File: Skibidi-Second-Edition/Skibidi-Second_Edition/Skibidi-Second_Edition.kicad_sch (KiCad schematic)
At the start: 72 parts, among them IC1 TEENSY_4.1, J1 Screw_Terminal_01x03, J10 Screw_Terminal_01x03, J11 Screw_Terminal_01x03, J12 12V, J13 Conn_01x03_Pin, J14 Conn_01x08_Pin, J15 Conn_02x05_Odd_Even, J16 P78E05-1000, J17 Conn_01x04_Pin, J2 Screw_Terminal_01x03, J3 Screw_Terminal_01x03, J4 Screw_Terminal_01x03, J5 Screw_Terminal_01x03, J6 Screw_Terminal_01x03, J7 Screw_Terminal_01x03, J8 Screw_Terminal_01x03, J9 Screw_Terminal_01x03, SW1 SW_Nidec_CAS-120A1, SW2 210-4MS

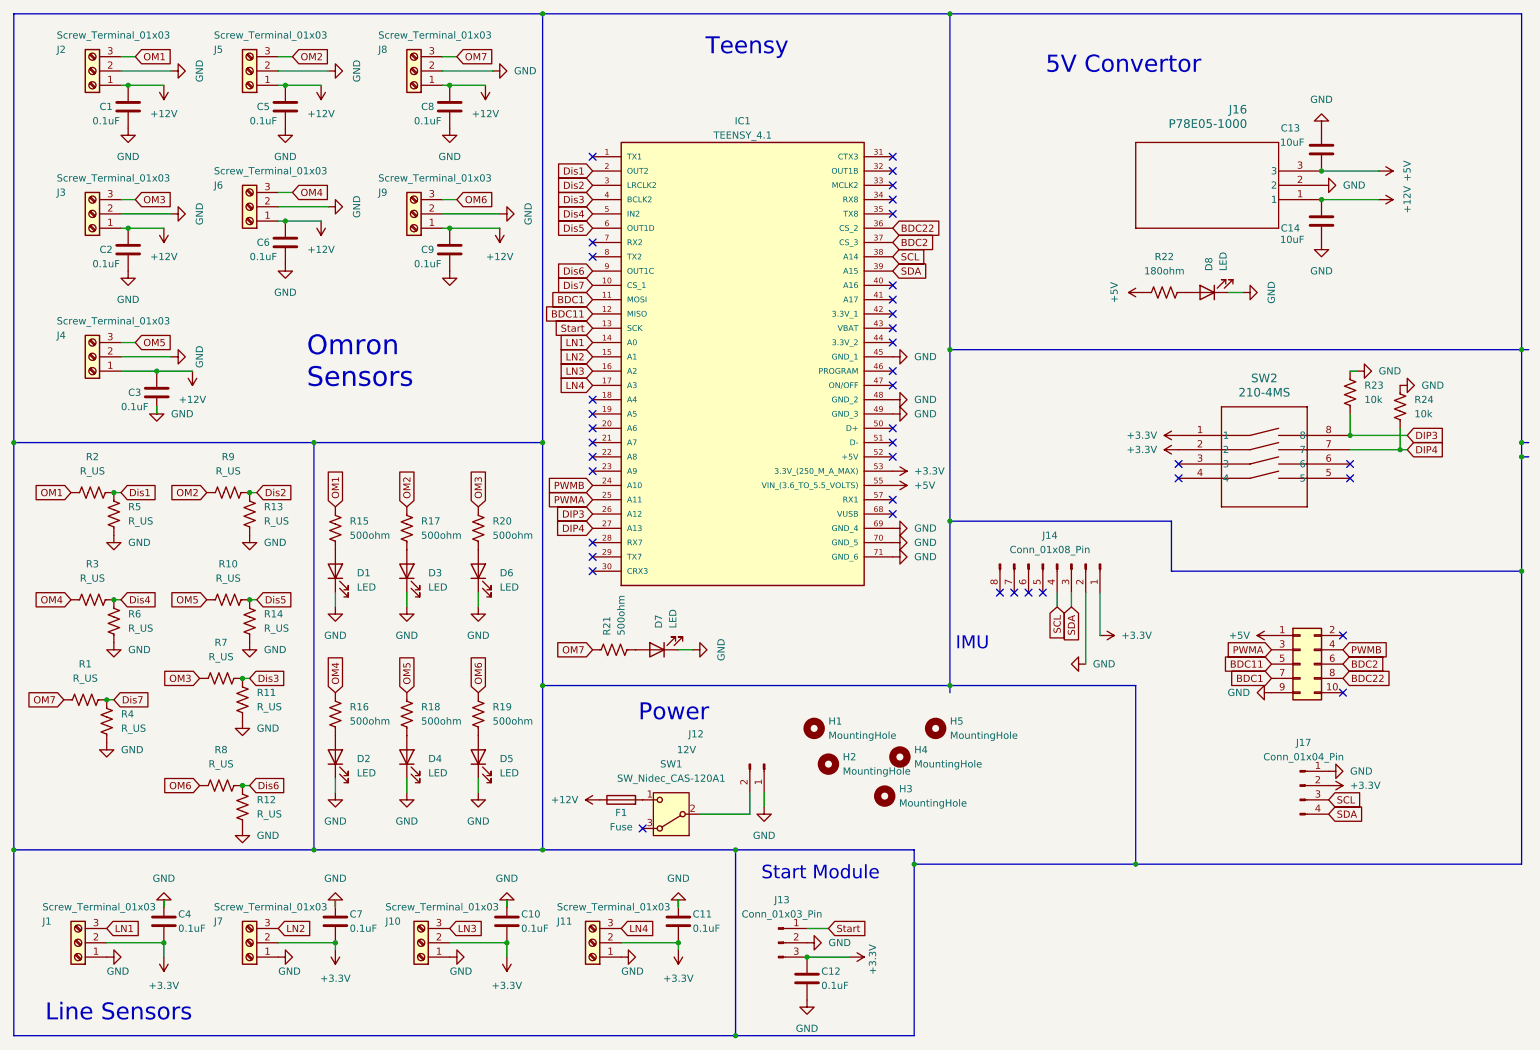
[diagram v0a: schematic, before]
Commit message: skibidi
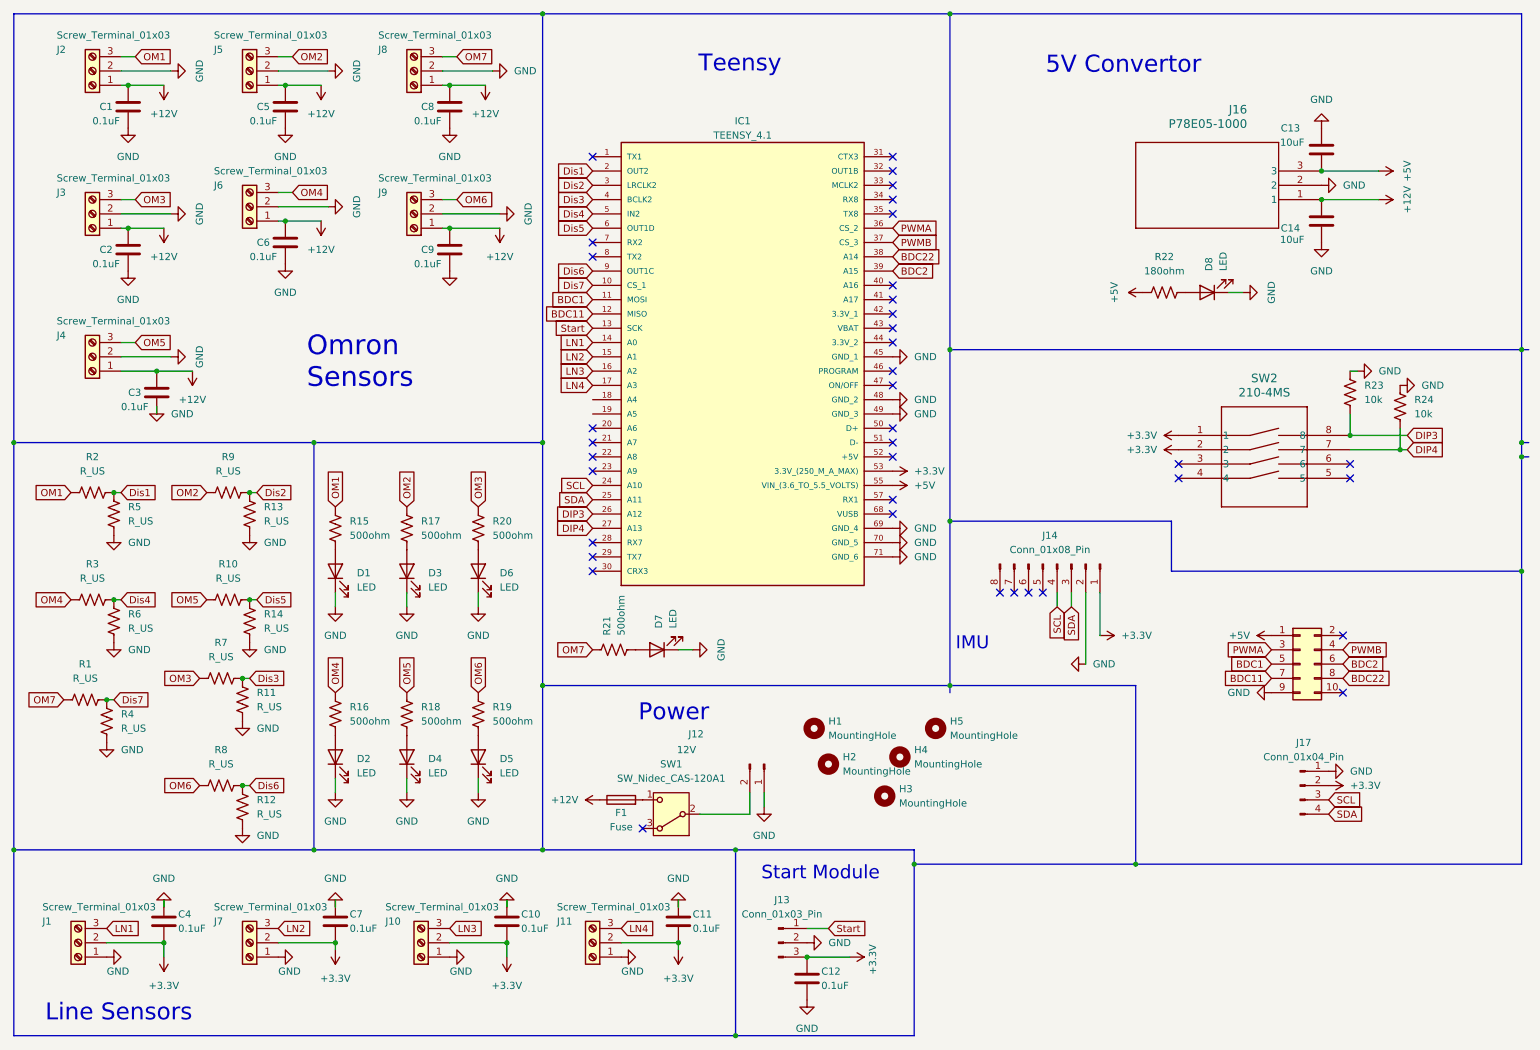
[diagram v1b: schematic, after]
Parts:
- J1, J10, J11, J2, J3, J4, J5, J6, J7, J8, J9: footprint TerminalBlock:TerminalBlock_Xinya_XY308-2.54-3P_1x03_P2.54mm_Horizontal -> Connector_JST:JST_EH_B3B-EH-A_1x03_P2.50mm_Vertical
- J17: footprint (none) -> Connector_PinHeader_2.54mm:PinHeader_1x04_P2.54mm_Vertical
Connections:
- net BDC1: now also J15.5 (Pin_5); no longer J15.7 (Pin_7)
- net BDC11: now also J15.7 (Pin_7); no longer J15.5 (Pin_5)
- net BDC2: now also IC1.39 (A15); no longer IC1.37 (CS_3)
- net BDC22: now also IC1.38 (A14); no longer IC1.36 (CS_2)
- net PWMA: now also IC1.36 (CS_2); no longer IC1.25 (A11)
- net PWMB: now also IC1.37 (CS_3); no longer IC1.24 (A10)
- net SCL: now also IC1.24 (A10); no longer IC1.38 (A14)
- net SDA: now also IC1.25 (A11); no longer IC1.39 (A15)
- no-connect marks 40 -> 38
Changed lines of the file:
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@@
 	)
 	(no_connect
-		(at 118.11 83.82)
-	)
-	(no_connect
 		(at 171.45 63.5)
 	)
@@
 	)
 	(no_connect
-		(at 118.11 81.28)
-	)
-	(no_connect
 		(at 118.11 53.34)
 	)
@@
 	(text "Teensy\n"
 		(exclude_from_sim no)
-		(at 138.176 20.32 0)
+		(at 136.906 23.368 0)
 		(effects
 			(font
@@
 		)
 	)
+	(global_label "PWMB"
+		(shape input)
+		(at 171.45 53.34 0)
+		(fields_autoplaced yes)
+		(effects
+			(font
+				(size 1.27 1.27)
+			)
+			(justify left)
+		)
+		(property "Intersheetrefs" "${INTERSHEET_REFS}"
+			(at 179.878 53.34 0)
+			(effects
+				(font
+					(size 1.27 1.27)
+				)
+				(justify left)
+				(hide yes)
+			)
+		)
+	)
 	(global_label "Dis1"
 		(shape input)
@@
 		)
 	)
+	(global_label "PWMA"
+		(shape input)
+		(at 171.45 50.8 0)
+		(fields_autoplaced yes)
+		(effects
+			(font
+				(size 1.27 1.27)
+			)
+			(justify left)
+		)
+		(property "Intersheetrefs" "${INTERSHEET_REFS}"
+			(at 179.6966 50.8 0)
+			(effects
+				(font
+					(size 1.27 1.27)
+				)
+				(justify left)
+				(hide yes)
+			)
+		)
+	)
+	(global_label "SCL"
+		(shape input)
+		(at 118.11 96.52 180)
+		(fields_autoplaced yes)
+		(effects
+			(font
+				(size 1.27 1.27)
+			)
+			(justify right)
+		)
+		(property "Intersheetrefs" "${INTERSHEET_REFS}"
+			(at 111.6172 96.52 0)
+			(effects
+				(font
+					(size 1.27 1.27)
+				)
+				(justify right)
+				(hide yes)
+			)
+		)
+	)
 	(global_label "SCL"
 		(shape input)
@@
 		)
 	)
-	(global_label "BDC2"
-		(shape input)
-		(at 171.45 53.34 0)
-		(fields_autoplaced yes)
-		(effects
-			(font
-				(size 1.27 1.27)
-			)
-			(justify left)
-		)
-		(property "Intersheetrefs" "${INTERSHEET_REFS}"
-			(at 179.4547 53.34 0)
-			(effects
-				(font
-					(size 1.27 1.27)
-				)
-				(justify left)
-				(hide yes)
-			)
-		)
-	)
 	(global_label "Dis4"
 		(shape input)
@@
 		)
 	)
-	(global_label "BDC11"
+	(global_label "BDC1"
 		(shape input)
 		(at 238.76 128.27 180)
@@
 		)
 		(property "Intersheetrefs" "${INTERSHEET_REFS}"
-			(at 229.5458 128.27 0)
+			(at 230.7553 128.27 0)
 			(effects
 				(font
@@
 		)
 	)
-	(global_label "BDC1"
+	(global_label "BDC11"
 		(shape input)
 		(at 238.76 130.81 180)
@@
 		)
 		(property "Intersheetrefs" "${INTERSHEET_REFS}"
-			(at 230.7553 130.81 0)
+			(at 229.5458 130.81 0)
 			(effects
 				(font
@@
 		)
 	)
-	(global_label "BDC22"
+	(global_label "LN2"
 		(shape input)
-		(at 171.45 50.8 0)
+		(at 62.23 175.26 0)
 		(fields_autoplaced yes)
 		(effects
@@
 		)
 		(property "Intersheetrefs" "${INTERSHEET_REFS}"
-			(at 180.6642 50.8 0)
+			(at 68.7833 175.26 0)
 			(effects
 				(font
@@
 		)
 	)
-	(global_label "PWMB"
-		(shape input)
-		(at 118.11 96.52 180)
-		(fields_autoplaced yes)
-		(effects
-			(font
-				(size 1.27 1.27)
-			)
-			(justify right)
-		)
-		(property "Intersheetrefs" "${INTERSHEET_REFS}"
-			(at 109.682 96.52 0)
-			(effects
-				(font
-					(size 1.27 1.27)
-				)
-				(justify right)
-				(hide yes)
-			)
-		)
-	)
-	(global_label "LN2"
+	(global_label "BDC2"
 		(shape input)
-		(at 62.23 175.26 0)
+		(at 171.45 58.42 0)
 		(fields_autoplaced yes)
 		(effects
@@
 		)
 		(property "Intersheetrefs" "${INTERSHEET_REFS}"
-			(at 68.7833 175.26 0)
+			(at 179.4547 58.42 0)
 			(effects
 				(font
@@
 		)
 	)
-	(global_label "SCL"
+	(global_label "DIP4"
 		(shape input)
-		(at 171.45 55.88 0)
+		(at 118.11 104.14 180)
 		(fields_autoplaced yes)
 		(effects
@@
 				(size 1.27 1.27)
 			)
-			(justify left)
+			(justify right)
 		)
 		(property "Intersheetrefs" "${INTERSHEET_REFS}"
-			(at 177.9428 55.88 0)
+			(at 110.7705 104.14 0)
 			(effects
 				(font
 					(size 1.27 1.27)
 				)
-				(justify left)
+				(justify right)
 				(hide yes)
 			)
 		)
 	)
-	(global_label "DIP4"
+	(global_label "SDA"
 		(shape input)
-		(at 118.11 104.14 180)
+		(at 203.2 118.11 270)
 		(fields_autoplaced yes)
 		(effects
@@
 		)
 		(property "Intersheetrefs" "${INTERSHEET_REFS}"
-			(at 110.7705 104.14 0)
+			(at 203.2 124.6633 90)
 			(effects
 				(font
@@
 		)
 	)
-	(global_label "SDA"
+	(global_label "BDC22"
 		(shape input)
-		(at 203.2 118.11 270)
+		(at 171.45 55.88 0)
 		(fields_autoplaced yes)
 		(effects
@@
 				(size 1.27 1.27)
 			)
-			(justify right)
+			(justify left)
 		)
 		(property "Intersheetrefs" "${INTERSHEET_REFS}"
-			(at 203.2 124.6633 90)
+			(at 180.6642 55.88 0)
 			(effects
 				(font
 					(size 1.27 1.27)
 				)
-				(justify right)
+				(justify left)
 				(hide yes)
 			)
@@
 		)
 	)
-	(global_label "PWMA"
-		(shape input)
-		(at 118.11 99.06 180)
-		(fields_autoplaced yes)
-		(effects
-			(font
-				(size 1.27 1.27)
-			)
-			(justify right)
-		)
-		(property "Intersheetrefs" "${INTERSHEET_REFS}"
-			(at 109.8634 99.06 0)
-			(effects
-				(font
-					(size 1.27 1.27)
-				)
-				(justify right)
-				(hide yes)
-			)
-		)
-	)
 	(global_label "Dis2"
 		(shape input)
@@
 		)
 	)
-	(global_label "SDA"
-		(shape input)
-		(at 171.45 58.42 0)
-		(fields_autoplaced yes)
-		(effects
-			(font
-				(size 1.27 1.27)
-			)
-			(justify left)
-		)
-		(property "Intersheetrefs" "${INTERSHEET_REFS}"
-			(at 178.0033 58.42 0)
-			(effects
-				(font
-					(size 1.27 1.27)
-				)
-				(justify left)
-				(hide yes)
-			)
-		)
-	)
 	(global_label "OM3"
 		(shape input)
@@
 		)
 	)
+	(global_label "SDA"
+		(shape input)
+		(at 118.11 99.06 180)
+		(fields_autoplaced yes)
+		(effects
+			(font
+				(size 1.27 1.27)
+			)
+			(justify right)
+		)
+		(property "Intersheetrefs" "${INTERSHEET_REFS}"
+			(at 111.5567 99.06 0)
+			(effects
+				(font
+					(size 1.27 1.27)
+				)
+				(justify right)
+				(hide yes)
+			)
+		)
+	)
 	(global_label "BDC2"
 		(shape input)
@@
 			)
 		)
-		(property "Footprint" "TerminalBlock:TerminalBlock_Xinya_XY308-2.54-3P_1x03_P2.54mm_Horizontal"
+		(property "Footprint" "Connector_JST:JST_EH_B3B-EH-A_1x03_P2.50mm_Vertical"
 			(at 118.11 177.8 0)
 			(effects
@@
 			)
 		)
-		(property "Footprint" "TerminalBlock:TerminalBlock_Xinya_XY308-2.54-3P_1x03_P2.54mm_Horizontal"
+		(property "Footprint" "Connector_JST:JST_EH_B3B-EH-A_1x03_P2.50mm_Vertical"
 			(at 86.36 48.26 0)
 			(effects
@@
 			)
 		)
-		(property "Footprint" "TerminalBlock:TerminalBlock_Xinya_XY308-2.54-3P_1x03_P2.54mm_Horizontal"
+		(property "Footprint" "Connector_JST:JST_EH_B3B-EH-A_1x03_P2.50mm_Vertical"
 			(at 26.67 177.8 0)
 			(effects
@@
 			)
 		)
-		(property "Footprint" "TerminalBlock:TerminalBlock_Xinya_XY308-2.54-3P_1x03_P2.54mm_Horizontal"
+		(property "Footprint" "Connector_JST:JST_EH_B3B-EH-A_1x03_P2.50mm_Vertical"
 			(at 29.21 73.66 0)
 			(effects
@@
 			)
 		)
-		(property "Footprint" ""
+		(property "Footprint" "Connector_PinHeader_2.54mm:PinHeader_1x04_P2.54mm_Vertical"
 			(at 243.84 149.86 0)
 			(effects
@@
 			)
 		)
-		(property "Footprint" "TerminalBlock:TerminalBlock_Xinya_XY308-2.54-3P_1x03_P2.54mm_Horizontal"
+		(property "Footprint" "Connector_JST:JST_EH_B3B-EH-A_1x03_P2.50mm_Vertical"
 			(at 87.63 177.8 0)
 			(effects
@@
 			)
 		)
-		(property "Footprint" "TerminalBlock:TerminalBlock_Xinya_XY308-2.54-3P_1x03_P2.54mm_Horizontal"
+		(property "Footprint" "Connector_JST:JST_EH_B3B-EH-A_1x03_P2.50mm_Vertical"
 			(at 57.15 46.99 0)
 			(effects
@@
 			)
 		)
-		(property "Footprint" "TerminalBlock:TerminalBlock_Xinya_XY308-2.54-3P_1x03_P2.54mm_Horizontal"
+		(property "Footprint" "Connector_JST:JST_EH_B3B-EH-A_1x03_P2.50mm_Vertical"
 			(at 57.15 177.8 0)
 			(effects
@@
 			)
 		)
-		(property "Footprint" "TerminalBlock:TerminalBlock_Xinya_XY308-2.54-3P_1x03_P2.54mm_Horizontal"
+		(property "Footprint" "Connector_JST:JST_EH_B3B-EH-A_1x03_P2.50mm_Vertical"
 			(at 29.21 22.86 0)
 			(effects
@@
 			)
 		)
-		(property "Footprint" "TerminalBlock:TerminalBlock_Xinya_XY308-2.54-3P_1x03_P2.54mm_Horizontal"
+		(property "Footprint" "Connector_JST:JST_EH_B3B-EH-A_1x03_P2.50mm_Vertical"
 			(at 57.15 22.86 0)
 			(effects
@@
 			)
 		)
-		(property "Footprint" "TerminalBlock:TerminalBlock_Xinya_XY308-2.54-3P_1x03_P2.54mm_Horizontal"
+		(property "Footprint" "Connector_JST:JST_EH_B3B-EH-A_1x03_P2.50mm_Vertical"
 			(at 29.21 48.26 0)
 			(effects
@@
 			)
 		)
-		(property "Footprint" "TerminalBlock:TerminalBlock_Xinya_XY308-2.54-3P_1x03_P2.54mm_Horizontal"
+		(property "Footprint" "Connector_JST:JST_EH_B3B-EH-A_1x03_P2.50mm_Vertical"
 			(at 86.36 22.86 0)
 			(effects

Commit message: bobbi
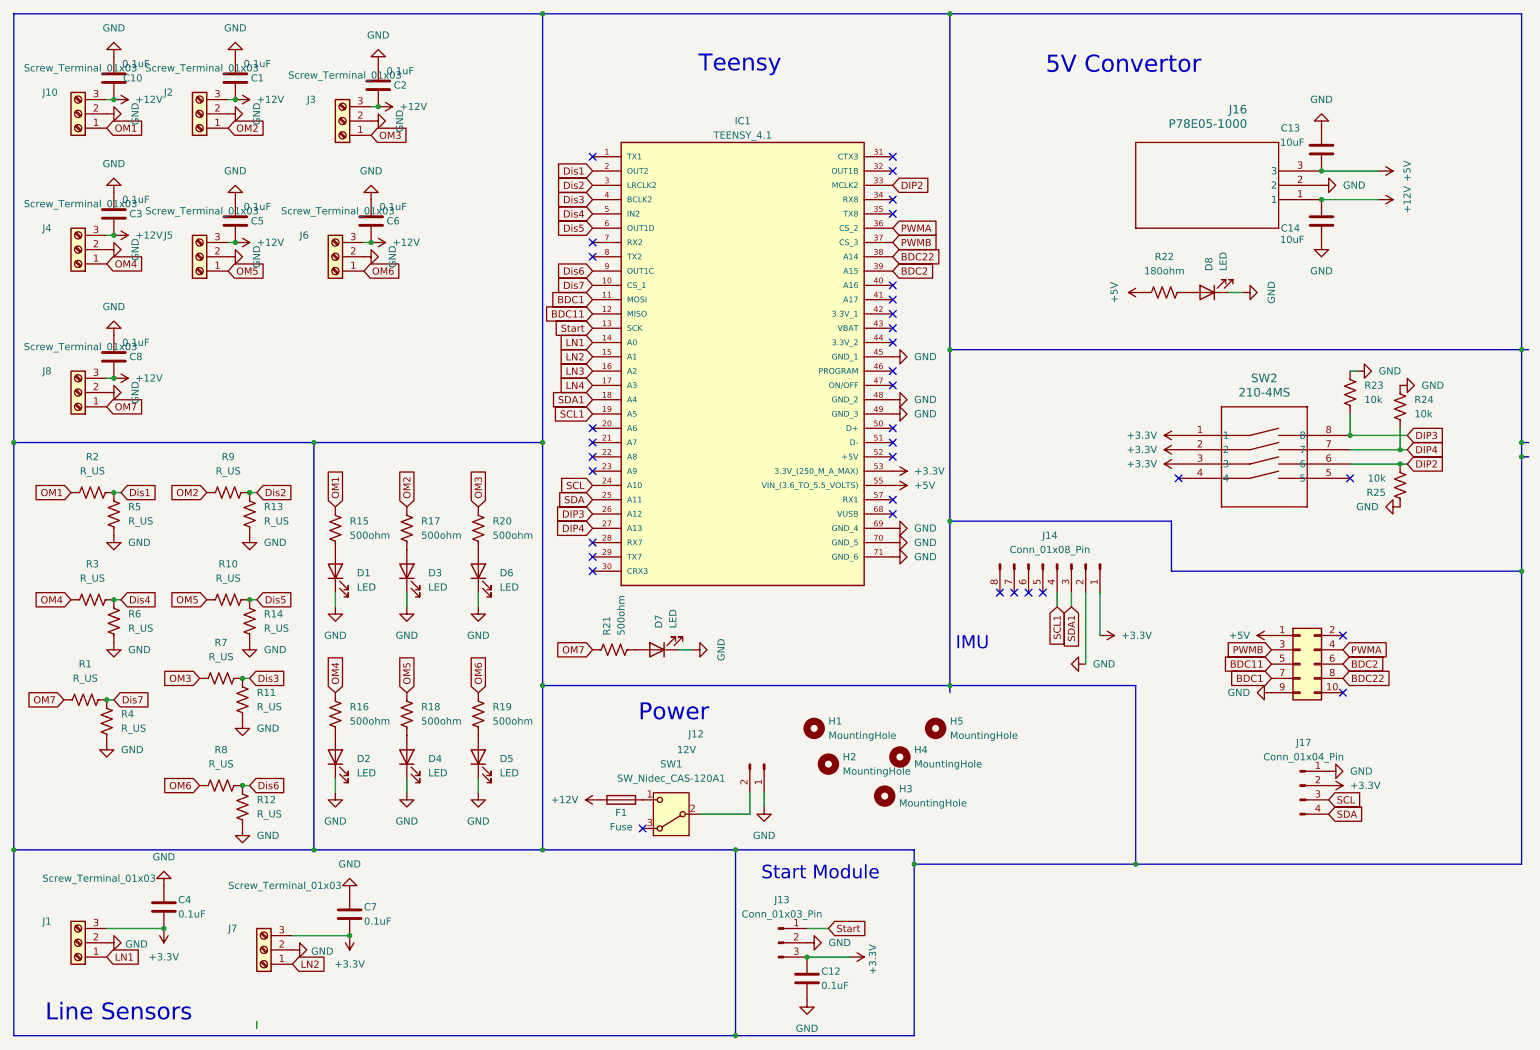
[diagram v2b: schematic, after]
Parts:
- removed C11, C9: 0.1uF, Capacitor_SMD:C_0805_2012Metric, symbol Device:C
- removed J11, J9: Screw_Terminal_01x03, Connector_JST:JST_EH_B3B-EH-A_1x03_P2.50mm_Vertical, symbol Connector:Screw_Terminal_01x03
- added R25: 10k, Capacitor_SMD:C_1206_3216Metric, symbol Device:R_US
- J1, J10, J2, J3, J4, J5, J6, J7, J8: footprint Connector_JST:JST_EH_B3B-EH-A_1x03_P2.50mm_Vertical -> Connector_JST:JST_PH_B3B-PH-K_1x03_P2.00mm_Vertical
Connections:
- net +12V: now also C10.1, J10.3 (Pin_3), J2.3 (Pin_3), J3.3 (Pin_3), J4.3 (Pin_3), J5.3 (Pin_3), J6.3 (Pin_3), J8.3 (Pin_3); no longer J2.1 (Pin_1), J3.1 (Pin_1), J4.1 (Pin_1), J5.1 (Pin_1), J6.1 (Pin_1), J8.1 (Pin_1)
- net +3.3V: now also J1.3 (Pin_3), J7.3 (Pin_3), SW2.3; no longer C10.2, J1.2 (Pin_2), J10.2 (Pin_2), J7.2 (Pin_2)
- net BDC1: now also J15.7 (Pin_7); no longer J15.5 (Pin_5)
- net BDC11: now also J15.5 (Pin_5); no longer J15.7 (Pin_7)
- net GND: now also C10.2, J1.2 (Pin_2), J10.2 (Pin_2), J7.2 (Pin_2), R25.2; no longer C10.1, J1.1 (Pin_1), J10.1 (Pin_1), J7.1 (Pin_1)
- net LN1: now also J1.1 (Pin_1); no longer J1.3 (Pin_3)
- net LN2: now also J7.1 (Pin_1); no longer J7.3 (Pin_3)
- net LN3: no longer J10.3 (Pin_3)
- net OM1: now also J10.1 (Pin_1); no longer J2.3 (Pin_3)
- net OM2: now also J2.1 (Pin_1); no longer J5.3 (Pin_3)
- net OM3: now also J3.1 (Pin_1); no longer J3.3 (Pin_3)
- net OM4: now also J4.1 (Pin_1); no longer J6.3 (Pin_3)
- net OM5: now also J5.1 (Pin_1); no longer J4.3 (Pin_3)
- net OM6: now also J6.1 (Pin_1)
- net OM7: now also J8.1 (Pin_1); no longer J8.3 (Pin_3)
- net PWMA: now also J15.4 (Pin_4); no longer J15.3 (Pin_3)
- net PWMB: now also J15.3 (Pin_3); no longer J15.4 (Pin_4)
- net SCL: no longer J14.4 (Pin_4)
- net SDA: no longer J14.3 (Pin_3)
- net DIP2: now reaches SW2.6
- net DIP2: now also IC1.33 (MCLK2), R25.1
- net SDA1: now reaches IC1.18 (A4)
- net SDA1: now also J14.3 (Pin_3)
- net SCL1: now reaches IC1.19 (A5)
- net SCL1: now also J14.4 (Pin_4)
- no-connect marks 38 -> 35
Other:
- note removed: "Omron Sensors"
